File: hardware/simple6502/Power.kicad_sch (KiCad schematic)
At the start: 23 parts, among them J4 GND, J5 POWER 5V, J6 AUX 5VDC, SW2 POWER, U5 74HCT00, U6 74LS30, U7 74HCT273

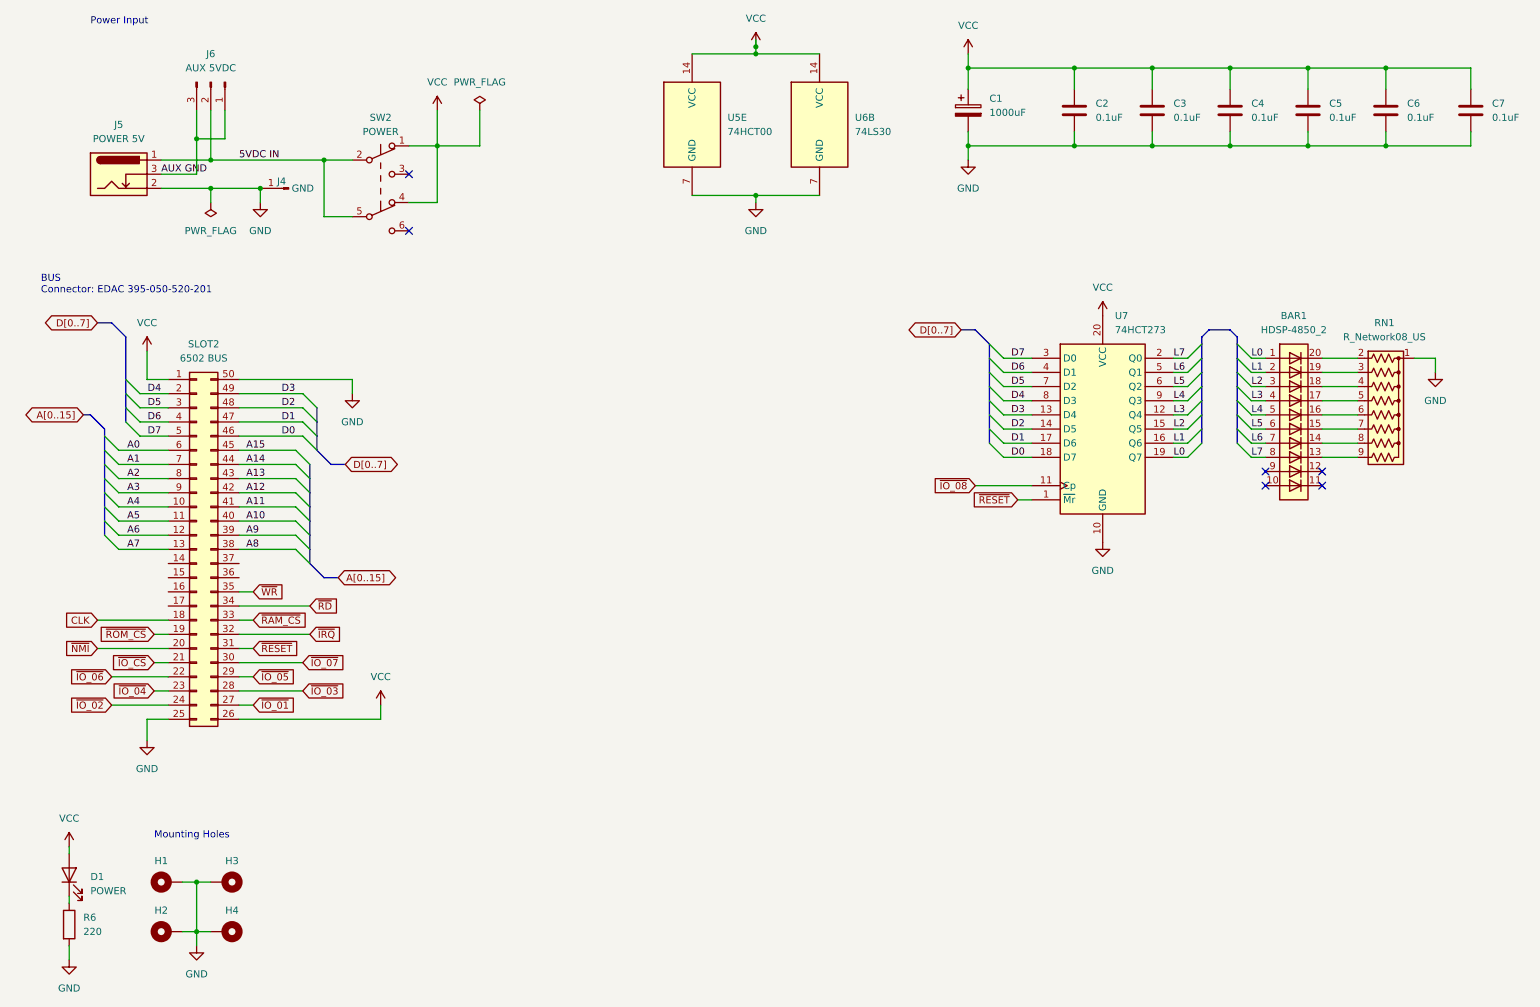
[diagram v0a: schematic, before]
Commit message: cpu board only ready
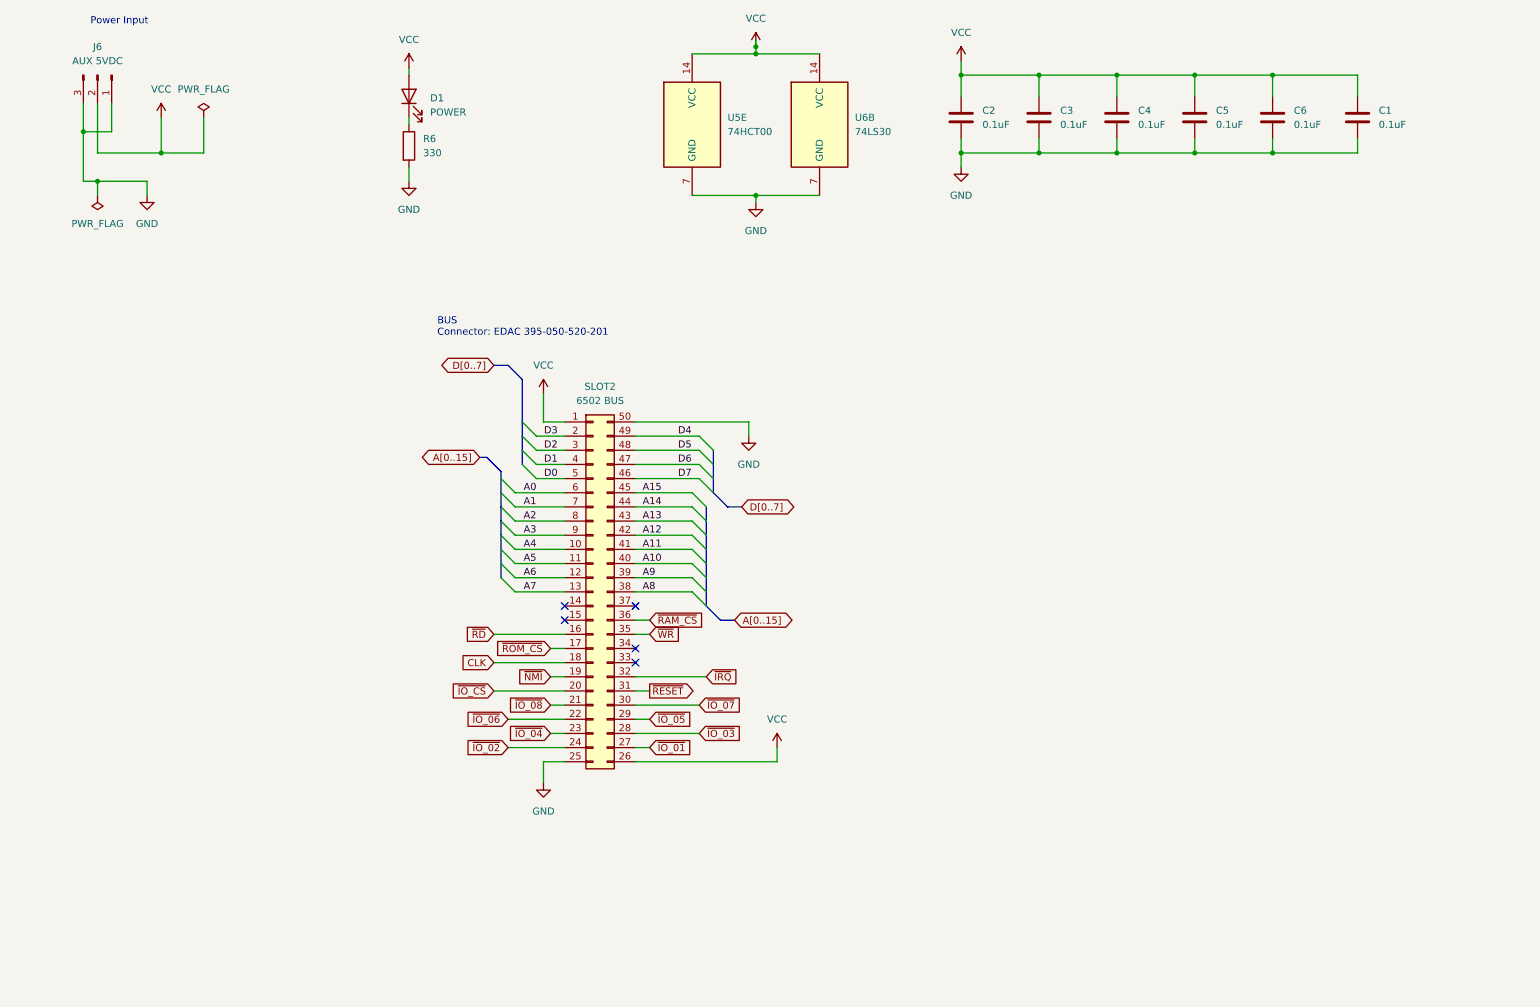
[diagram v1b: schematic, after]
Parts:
- removed BAR1: HDSP-4850_2, Display:HDSP-4850, symbol LED:HDSP-4850_2
- removed C1: 1000uF, Capacitor_THT:CP_Radial_D6.3mm_P2.50mm, symbol Device:C_Polarized
- removed H1, H2, H3, H4: M, MountingHole:MountingHole_2.7mm_M2.5_Pad_Via, symbol Mechanical:MountingHole_Pad
- removed J4: GND, Connector_PinHeader_2.54mm:PinHeader_1x01_P2.54mm_Vertical, symbol Connector:Conn_01x01_Pin
- removed J5: POWER 5V, Connector_BarrelJack:BarrelJack_Horizontal, symbol Connector:Barrel_Jack_Switch
- removed RN1: R_Network08_US, Resistor_THT:R_Array_SIP9, symbol Device:R_Network08_US
- removed SW2: POWER, Button_Switch_THT:SW_Push_2P2T_Toggle_CK_PVA2OAH5xxxxxxV2, symbol Switch:SW_Push_DPDT
- removed U7: 74HCT273, Package_DIP:DIP-20_W7.62mm_Socket, symbol 74xx:74HCT273
- R6: value 220 -> 330
- renumbered C7 to C1
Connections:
- net 5VDC IN is gone; now on net VCC: J6.2 (Pin_2)
- net AUX GND is gone; now on net GND: J6.1 (Pin_1), J6.3 (Pin_3)
- net D0: now also SLOT2.5 (Pin_5); no longer SLOT2.46 (Pin_46)
- net D1: now also SLOT2.4 (Pin_4); no longer SLOT2.47 (Pin_47)
- net D2: now also SLOT2.3 (Pin_3); no longer SLOT2.48 (Pin_48)
- net D3: now also SLOT2.2 (Pin_2); no longer SLOT2.49 (Pin_49)
- net D4: now also SLOT2.49 (Pin_49); no longer SLOT2.2 (Pin_2)
- net D5: now also SLOT2.48 (Pin_48); no longer SLOT2.3 (Pin_3)
- net D6: now also SLOT2.47 (Pin_47); no longer SLOT2.4 (Pin_4)
- net D7: now also SLOT2.46 (Pin_46); no longer SLOT2.5 (Pin_5)
- net ~{IO_08}: now also SLOT2.21 (Pin_21)
- net ~{IO_CS}: now also SLOT2.20 (Pin_20); no longer SLOT2.21 (Pin_21)
- net ~{NMI}: now also SLOT2.19 (Pin_19); no longer SLOT2.20 (Pin_20)
- net ~{RAM_CS}: now also SLOT2.36 (Pin_36); no longer SLOT2.33 (Pin_33)
- net ~{RD}: now also SLOT2.16 (Pin_16); no longer SLOT2.34 (Pin_34)
- net ~{ROM_CS}: now also SLOT2.17 (Pin_17); no longer SLOT2.19 (Pin_19)
- no-connect marks 6 -> 5
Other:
- note removed: "Mounting Holes"
- moved on the sheet: C1, C2, C3, C4, C5, C6, D1, J6, R6, SLOT2
